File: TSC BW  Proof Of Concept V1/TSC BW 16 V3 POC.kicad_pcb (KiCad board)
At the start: 2 copper layers, 177.4 x 113.6 mm, 232 parts, among them J1 691312510002, J10 Micro_SD_Card_Det_Hirose_DM3AT, J13 Analog Inputs, J14 USB_C_Receptacle_USB2.0_16P, J17 691312510002, J18 RJ45_Hanrun_HR911105A_Horizon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, J19 691312510002, J2 CR1220_S8411_45R, J3 Free GPIO !pull-up, J4 Free GPIO pull-up, J5 Terminal Plug, J7 Terminal Plug, Q1 BC817, Q10 NCE60P10K, Q11 NCE60P10K, Q14 NCE60P10K, Q15 NCE60P10K, Q18 NCE60P10K, Q19 NCE60P10K, Q2 AO3401A, Q20 SS8050, Q21 SS8050, Q6 NCE60P10K, Q7 NCE60P10K, SW1 SW_Push, SW2 SW_Push, U1 XL1509-5.0, U10 PC357C, U11 PC357C, U14 PC357C, U15 PC357C, U18 PC357C, U19 PC357C, U2 AMS1117-3.3, U20 PCF8574T, U24 PC357C, U25 PC357C, U28 PC357C, U29 PC357C, U3 ESP32-S3-WROOM-1, U32 PC357C, U33 PC357C, U36 PC357C, U37 PC357C, U38 PCF8574T, U40 AT24CS04-SSHM, U41 DS3231MZ, U44 CH340C, U46 W5500, U48 MAX13487EESA, U6 PC357C, U7 PC357C, Y4 25M

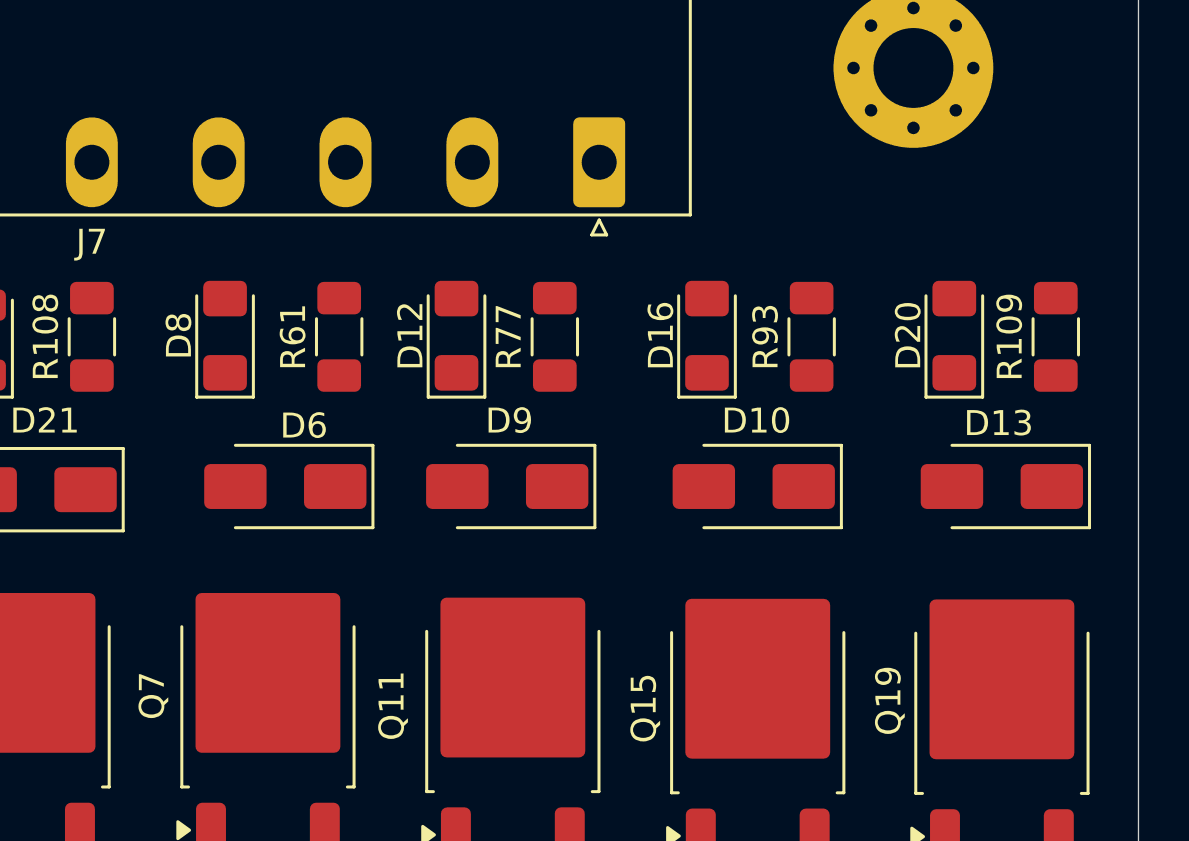
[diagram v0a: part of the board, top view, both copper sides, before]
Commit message: WORKING ON POC - Proof of concept
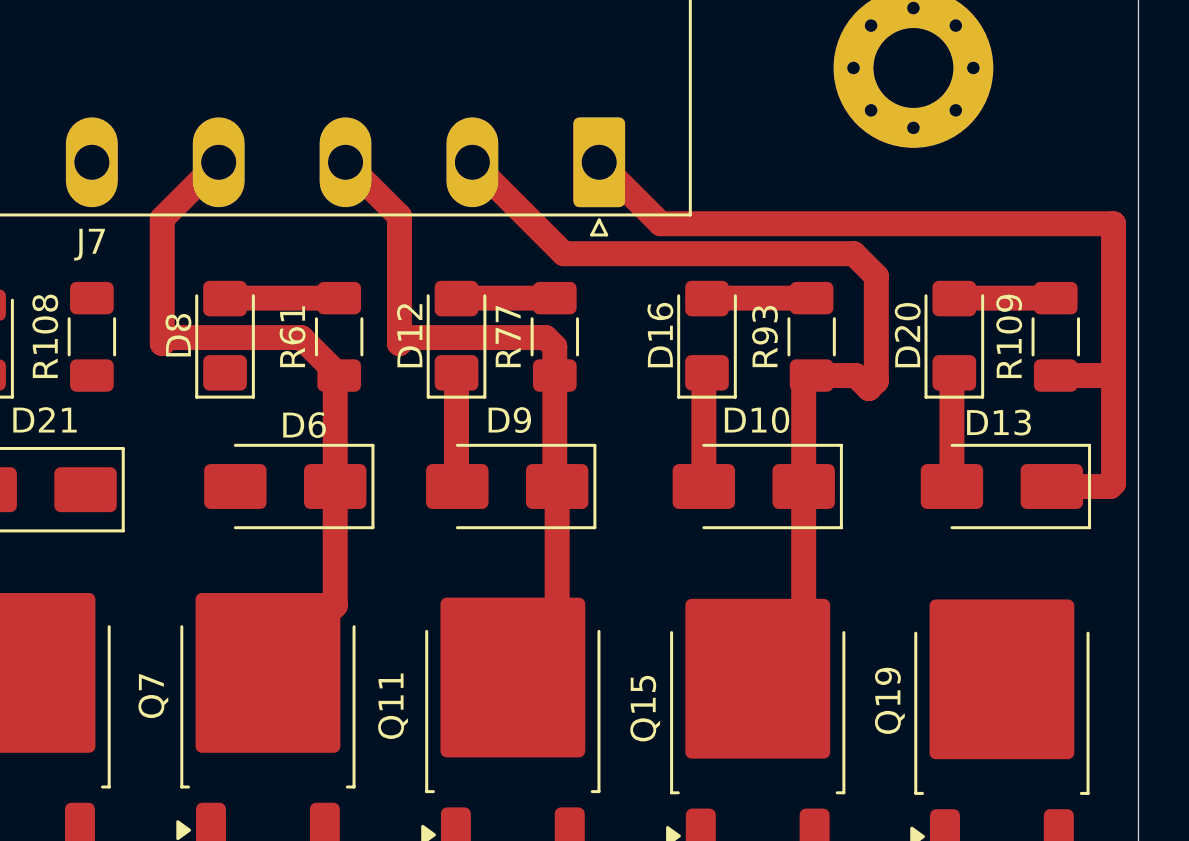
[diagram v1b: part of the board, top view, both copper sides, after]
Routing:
- net /8 DIGITAL OUTPUTS/outp7: track 0.00 -> 38.2 mm
- net /8 DIGITAL OUTPUTS/outp8: track 0.00 -> 36.9 mm
- net /8 DIGITAL OUTPUTS/outp5: track 0.00 -> 29.1 mm
- net /8 DIGITAL OUTPUTS/outp6: track 0.00 -> 28.7 mm
- net PGND: track 0.00 -> 13.8 mm
- net Net-(D8-A): track 0.00 -> 4.58 mm
- net Net-(D16-A): track 0.00 -> 4.20 mm
- net Net-(D20-A): track 0.00 -> 4.07 mm
- net Net-(D12-A): track 0.00 -> 3.94 mm
